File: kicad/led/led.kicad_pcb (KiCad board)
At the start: 2 copper layers, 73 x 25.1 mm, 45 parts, among them J1 Conn_01x06, J2 Conn_01x09_Male, U1 LF353DR, U2 LF353DR, U3 LF353DR, U4 LM339DR, U5 LM339DR

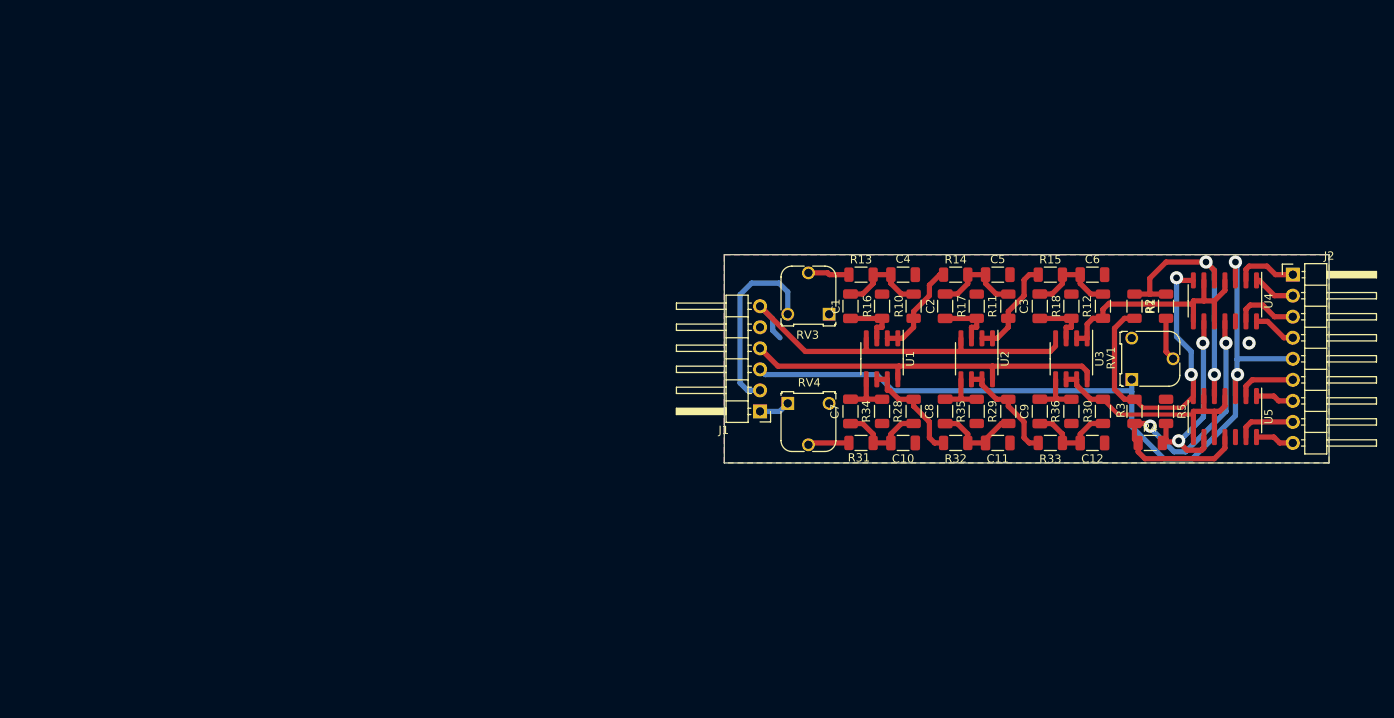
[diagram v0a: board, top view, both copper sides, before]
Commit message: Maybe finished LED board I think
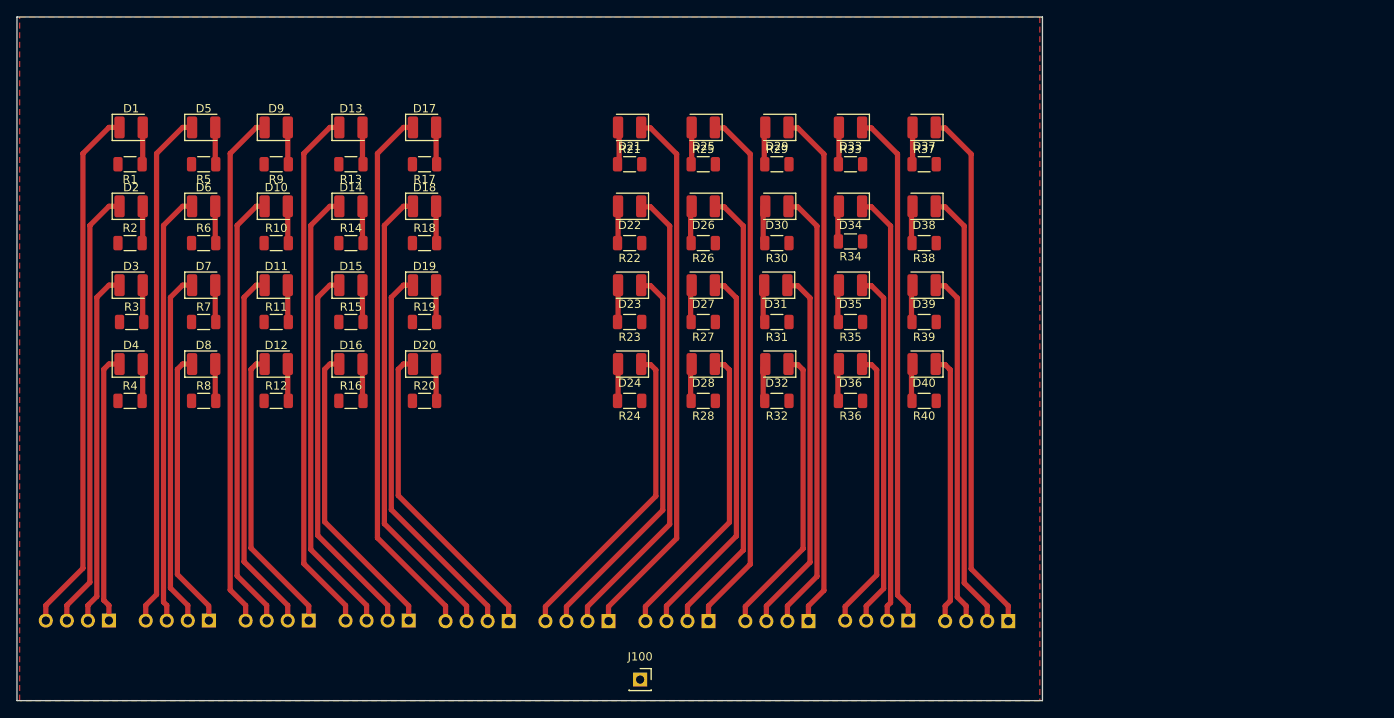
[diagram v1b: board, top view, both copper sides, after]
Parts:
- removed C1, C10, C11, C12, C2, C3, C4, C5, C6, C7, C8, C9: 100n, Capacitor_SMD:C_1206_3216Metric
- removed RV1, RV3, RV4: 10k, Potentiometer_THT:Potentiometer_Runtron_RM-065_Vertical
- removed U1, U2, U3: LF353DR, Package_SO:SOIC-8_3.9x4.9mm_P1.27mm
- removed U4, U5: LM339DR, Package_SO:SO-14_3.9x8.65mm_P1.27mm
- added D1: ORANGE, LED_SMD:LED_1210_3225Metric, F.Cu at (45.2, 46.4)
- added D10: YELLOW, LED_SMD:LED_1210_3225Metric, F.Cu at (62.7, 55.9)
- added D11: GREEN, LED_SMD:LED_1210_3225Metric, F.Cu at (62.7, 65.4)
- added D12: BLUE, LED_SMD:LED_1210_3225Metric, F.Cu at (62.7, 74.9)
- added D13: ORANGE, LED_SMD:LED_1210_3225Metric, F.Cu at (71.8, 46.4)
- added D14: YELLOW, LED_SMD:LED_1210_3225Metric, F.Cu at (71.8, 55.9)
- added D15: GREEN, LED_SMD:LED_1210_3225Metric, F.Cu at (71.8, 65.4)
- added D16: BLUE, LED_SMD:LED_1210_3225Metric, F.Cu at (71.8, 74.9)
- added D17: ORANGE, LED_SMD:LED_1210_3225Metric, F.Cu at (80.6, 46.4)
- added D18: YELLOW, LED_SMD:LED_1210_3225Metric, F.Cu at (80.6, 55.9)
- added D19: GREEN, LED_SMD:LED_1210_3225Metric, F.Cu at (80.6, 65.4)
- added D2: YELLOW, LED_SMD:LED_1210_3225Metric, F.Cu at (45.2, 55.9)
- added D20: BLUE, LED_SMD:LED_1210_3225Metric, F.Cu at (80.6, 74.9)
- added D21: ORANGE, LED_SMD:LED_1210_3225Metric, F.Cu at (105.4, 46.4)
- added D22: YELLOW, LED_SMD:LED_1210_3225Metric, F.Cu at (105.4, 55.9)
- added D23: GREEN, LED_SMD:LED_1210_3225Metric, F.Cu at (105.4, 65.4)
- added D24: BLUE, LED_SMD:LED_1210_3225Metric, F.Cu at (105.4, 74.9)
- added D25: ORANGE, LED_SMD:LED_1210_3225Metric, F.Cu at (114.3, 46.4)
- added D26: YELLOW, LED_SMD:LED_1210_3225Metric, F.Cu at (114.3, 55.9)
- added D27: GREEN, LED_SMD:LED_1210_3225Metric, F.Cu at (114.3, 65.4)
- added D28: BLUE, LED_SMD:LED_1210_3225Metric, F.Cu at (114.3, 74.9)
- added D29: ORANGE, LED_SMD:LED_1210_3225Metric, F.Cu at (123.2, 46.4)
- added D3: GREEN, LED_SMD:LED_1210_3225Metric, F.Cu at (45.2, 65.4)
- added D30: YELLOW, LED_SMD:LED_1210_3225Metric, F.Cu at (123.2, 55.9)
- added D31: GREEN, LED_SMD:LED_1210_3225Metric, F.Cu at (123.1, 65.4)
- added D32: BLUE, LED_SMD:LED_1210_3225Metric, F.Cu at (123.2, 74.9)
- added D33: ORANGE, LED_SMD:LED_1210_3225Metric, F.Cu at (132.1, 46.4)
- added D34: YELLOW, LED_SMD:LED_1210_3225Metric, F.Cu at (132.1, 55.9)
- added D35: GREEN, LED_SMD:LED_1210_3225Metric, F.Cu at (132.1, 65.4)
- added D36: BLUE, LED_SMD:LED_1210_3225Metric, F.Cu at (132.1, 74.9)
- added D37: ORANGE, LED_SMD:LED_1210_3225Metric, F.Cu at (141.0, 46.4)
- added D38: YELLOW, LED_SMD:LED_1210_3225Metric, F.Cu at (141.0, 55.9)
- added D39: GREEN, LED_SMD:LED_1210_3225Metric, F.Cu at (141.0, 65.4)
- added D4: BLUE, LED_SMD:LED_1210_3225Metric, F.Cu at (45.2, 74.9)
- added D40: BLUE, LED_SMD:LED_1210_3225Metric, F.Cu at (141.0, 74.9)
- added D5: ORANGE, LED_SMD:LED_1210_3225Metric, F.Cu at (54.0, 46.4)
- added D6: YELLOW, LED_SMD:LED_1210_3225Metric, F.Cu at (54.0, 55.9)
- added D7: GREEN, LED_SMD:LED_1210_3225Metric, F.Cu at (54.0, 65.4)
- added D8: BLUE, LED_SMD:LED_1210_3225Metric, F.Cu at (54.0, 74.9)
- added D9: ORANGE, LED_SMD:LED_1210_3225Metric, F.Cu at (62.7, 46.4)
- added J10: Conn_01x04_Male, Connector_PinHeader_2.54mm:PinHeader_1x04_P2.54mm_Horizontal, B.Cu at (151.1, 106.0)
- added J100: Conn_01x01_Male, Connector_PinSocket_2.54mm:PinSocket_1x01_P2.54mm_Vertical, F.Cu at (106.7, 113.0)
- added J3: Conn_01x04_Male, Connector_PinHeader_2.54mm:PinHeader_1x04_P2.54mm_Horizontal, B.Cu at (66.7, 105.9)
- added J4: Conn_01x04_Male, Connector_PinHeader_2.54mm:PinHeader_1x04_P2.54mm_Horizontal, B.Cu at (78.7, 105.9)
- added J5: Conn_01x04_Male, Connector_PinHeader_2.54mm:PinHeader_1x04_P2.54mm_Horizontal, B.Cu at (90.8, 106.0)
- added J6: Conn_01x04_Male, Connector_PinHeader_2.54mm:PinHeader_1x04_P2.54mm_Horizontal, B.Cu at (102.9, 106.0)
- added J7: Conn_01x04_Male, Connector_PinHeader_2.54mm:PinHeader_1x04_P2.54mm_Horizontal, B.Cu at (114.9, 106.0)
- added J8: Conn_01x04_Male, Connector_PinHeader_2.54mm:PinHeader_1x04_P2.54mm_Horizontal, B.Cu at (127.0, 106.0)
- added J9: Conn_01x04_Male, Connector_PinHeader_2.54mm:PinHeader_1x04_P2.54mm_Horizontal, B.Cu at (139.1, 105.9)
- added R19: R, Resistor_SMD:R_1206_3216Metric, F.Cu at (80.6, 69.8)
- added R20: R, Resistor_SMD:R_1206_3216Metric, F.Cu at (80.6, 79.4)
- added R21: R, Resistor_SMD:R_1206_3216Metric, F.Cu at (105.4, 50.8)
- added R22: R, Resistor_SMD:R_1206_3216Metric, F.Cu at (105.4, 60.3)
- added R23: R, Resistor_SMD:R_1206_3216Metric, F.Cu at (105.4, 69.8)
- added R24: R, Resistor_SMD:R_1206_3216Metric, F.Cu at (105.4, 79.4)
- added R25: R, Resistor_SMD:R_1206_3216Metric, F.Cu at (114.3, 50.8)
- added R26: R, Resistor_SMD:R_1206_3216Metric, F.Cu at (114.3, 60.3)
- added R27: R, Resistor_SMD:R_1206_3216Metric, F.Cu at (114.3, 69.8)
- added R37: R, Resistor_SMD:R_1206_3216Metric, F.Cu at (141.0, 50.8)
- added R38: R, Resistor_SMD:R_1206_3216Metric, F.Cu at (141.0, 60.3)
- added R39: R, Resistor_SMD:R_1206_3216Metric, F.Cu at (141.0, 69.8)
- added R40: R, Resistor_SMD:R_1206_3216Metric, F.Cu at (141.0, 79.4)
- added R6: R, Resistor_SMD:R_1206_3216Metric, F.Cu at (54.0, 60.3)
- added R7: R, Resistor_SMD:R_1206_3216Metric, F.Cu at (54.0, 69.8)
- added R8: R, Resistor_SMD:R_1206_3216Metric, F.Cu at (54.0, 79.4)
- added R9: R, Resistor_SMD:R_1206_3216Metric, F.Cu at (62.7, 50.8)
- J1: value Conn_01x06 -> Conn_01x04_Male; footprint Connector_PinHeader_2.54mm:PinHeader_1x06_P2.54mm_Horizontal -> Connector_PinHeader_2.54mm:PinHeader_1x04_P2.54mm_Horizontal; moved to B.Cu
- J2: value Conn_01x09_Male -> Conn_01x04_Male; footprint Connector_PinHeader_2.54mm:PinHeader_1x09_P2.54mm_Horizontal -> Connector_PinHeader_2.54mm:PinHeader_1x04_P2.54mm_Horizontal; moved to B.Cu
- R1, R2, R3, R4, R5: value 100k -> R
- R10, R11, R12, R28, R29, R30: value 137 -> R
- R13, R14, R15, R31, R32, R33: value 931 -> R
- R16, R17, R18, R34, R35, R36: value 1k87 -> R
- moved J2 137.4 mm to (54.6, 105.9), turned to 90 degrees
- moved R1 126.3 mm to (45.1, 50.8), turned to 180 degrees
- moved R4 123.3 mm to (45.1, 79.4)
- moved R3 121.6 mm to (45.3, 69.8), turned to 0 degrees
- moved R2 121.5 mm to (45.1, 60.3), turned to 0 degrees
- moved R5 120.0 mm to (54.0, 50.8), turned to 180 degrees
- moved R12 100.5 mm to (62.7, 79.4), turned to 0 degrees
- moved R11 88.4 mm to (62.7, 69.8), turned to 0 degrees
- moved R15 84.6 mm to (71.8, 69.8)
- moved J1 82.6 mm to (42.5, 105.9), turned to 90 degrees
- moved R18 78.5 mm to (80.6, 60.3), turned to 0 degrees
- moved R10 77.3 mm to (62.7, 60.3), turned to 0 degrees
- moved R14 73.1 mm to (71.8, 60.3)
- moved R17 68.8 mm to (80.6, 50.8), turned to 180 degrees
- moved R16 65.1 mm to (71.8, 79.4), turned to 0 degrees
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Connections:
- J1 pad 3: +5V -> Net-(D2-Pad1)
- J1 pad 4: +15V -> Net-(J1-Pad4)
- R1 pad 2: Net-(R1-Pad2) -> +5V
- R10 pad 1: Net-(C4-Pad1) -> +5V
- R10 pad 2: Net-(R10-Pad2) -> Net-(D10-Pad2)
- R11 pad 1: Net-(C5-Pad1) -> +5V
- R11 pad 2: Net-(R11-Pad2) -> Net-(D11-Pad2)
- R12 pad 1: Net-(C6-Pad1) -> +5V
- R13 pad 1: audio_left -> Net-(D13-Pad2)
- R13 pad 2: Net-(C4-Pad1) -> +5V
- R14 pad 1: Net-(R10-Pad2) -> +5V
- R14 pad 2: Net-(C5-Pad1) -> Net-(D14-Pad2)
- R15 pad 1: Net-(R11-Pad2) -> +5V
- R15 pad 2: Net-(C6-Pad1) -> Net-(D15-Pad2)
- R16 pad 1: Net-(C1-Pad2) -> +5V
- R16 pad 2: GND -> Net-(D16-Pad2)
- R17 pad 2: GND -> +5V
- R18 pad 1: Net-(C3-Pad2) -> +5V
- R18 pad 2: GND -> Net-(D18-Pad2)
- R2 pad 1: Net-(R1-Pad2) -> +5V
- R2 pad 2: Net-(R2-Pad2) -> Net-(D2-Pad2)
- R28 pad 1: Net-(C10-Pad1) -> +5V
- R28 pad 2: Net-(R28-Pad2) -> Net-(D28-Pad2)
- R29 pad 1: Net-(C11-Pad1) -> Net-(D29-Pad2)
- R29 pad 2: Net-(R29-Pad2) -> +5V
- R3 pad 1: Net-(R2-Pad2) -> +5V
- R3 pad 2: Net-(R3-Pad2) -> Net-(D3-Pad2)
- R30 pad 1: Net-(C12-Pad1) -> +5V
- R31 pad 1: audio_right -> +5V
- R31 pad 2: Net-(C10-Pad1) -> Net-(D31-Pad2)
- R32 pad 1: Net-(R28-Pad2) -> +5V
- R32 pad 2: Net-(C11-Pad1) -> Net-(D32-Pad2)
- R33 pad 1: Net-(R29-Pad2) -> Net-(D33-Pad2)
- R33 pad 2: Net-(C12-Pad1) -> +5V
- R34 pad 1: Net-(C7-Pad2) -> +5V
- R34 pad 2: GND -> Net-(D34-Pad2)
- R35 pad 1: Net-(C8-Pad2) -> +5V
- R35 pad 2: GND -> Net-(D35-Pad2)
- R36 pad 1: Net-(C9-Pad2) -> +5V
- R36 pad 2: GND -> Net-(D36-Pad2)
- R4 pad 1: Net-(R3-Pad2) -> +5V
- R4 pad 2: Net-(R4-Pad2) -> Net-(D4-Pad2)
- R5 pad 1: Net-(R4-Pad2) -> Net-(D5-Pad2)
- R5 pad 2: GND -> +5V
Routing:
- net +5V: track 98.4 -> 0.00 mm, vias 2 -> 0
- net Net-(D17-Pad1): track 0.00 -> 65.5 mm
- net Net-(D21-Pad1): track 0.00 -> 65.4 mm
- net Net-(D13-Pad1): track 0.00 -> 64.1 mm
- net Net-(D25-Pad1): track 0.00 -> 64.1 mm
- net Net-(J1-Pad4): track 0.00 -> 63.9 mm
- net Net-(D37-Pad1): track 0.00 -> 63.9 mm
- net Net-(D9-Pad1): track 0.00 -> 62.8 mm
- net Net-(D29-Pad1): track 0.00 -> 62.8 mm
- net Net-(D33-Pad1): track 0.00 -> 62.5 mm
- net Net-(D5-Pad1): track 5.21 -> 62.5 mm
- net Net-(D18-Pad1): track 0.00 -> 56.3 mm
- net Net-(D22-Pad1): track 0.00 -> 56.2 mm
- net Net-(D14-Pad1): track 0.00 -> 54.9 mm
- net Net-(D26-Pad1): track 0.00 -> 54.9 mm
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- added copper zone on F.Cu, net +5V
- removed copper zone on B.Cu, net GND
- removed copper zone on F.Cu, net GND
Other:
- board size 73 x 25.1 mm -> 123.8 x 82.5 mm
